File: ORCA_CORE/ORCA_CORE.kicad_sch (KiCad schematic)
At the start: 0 parts

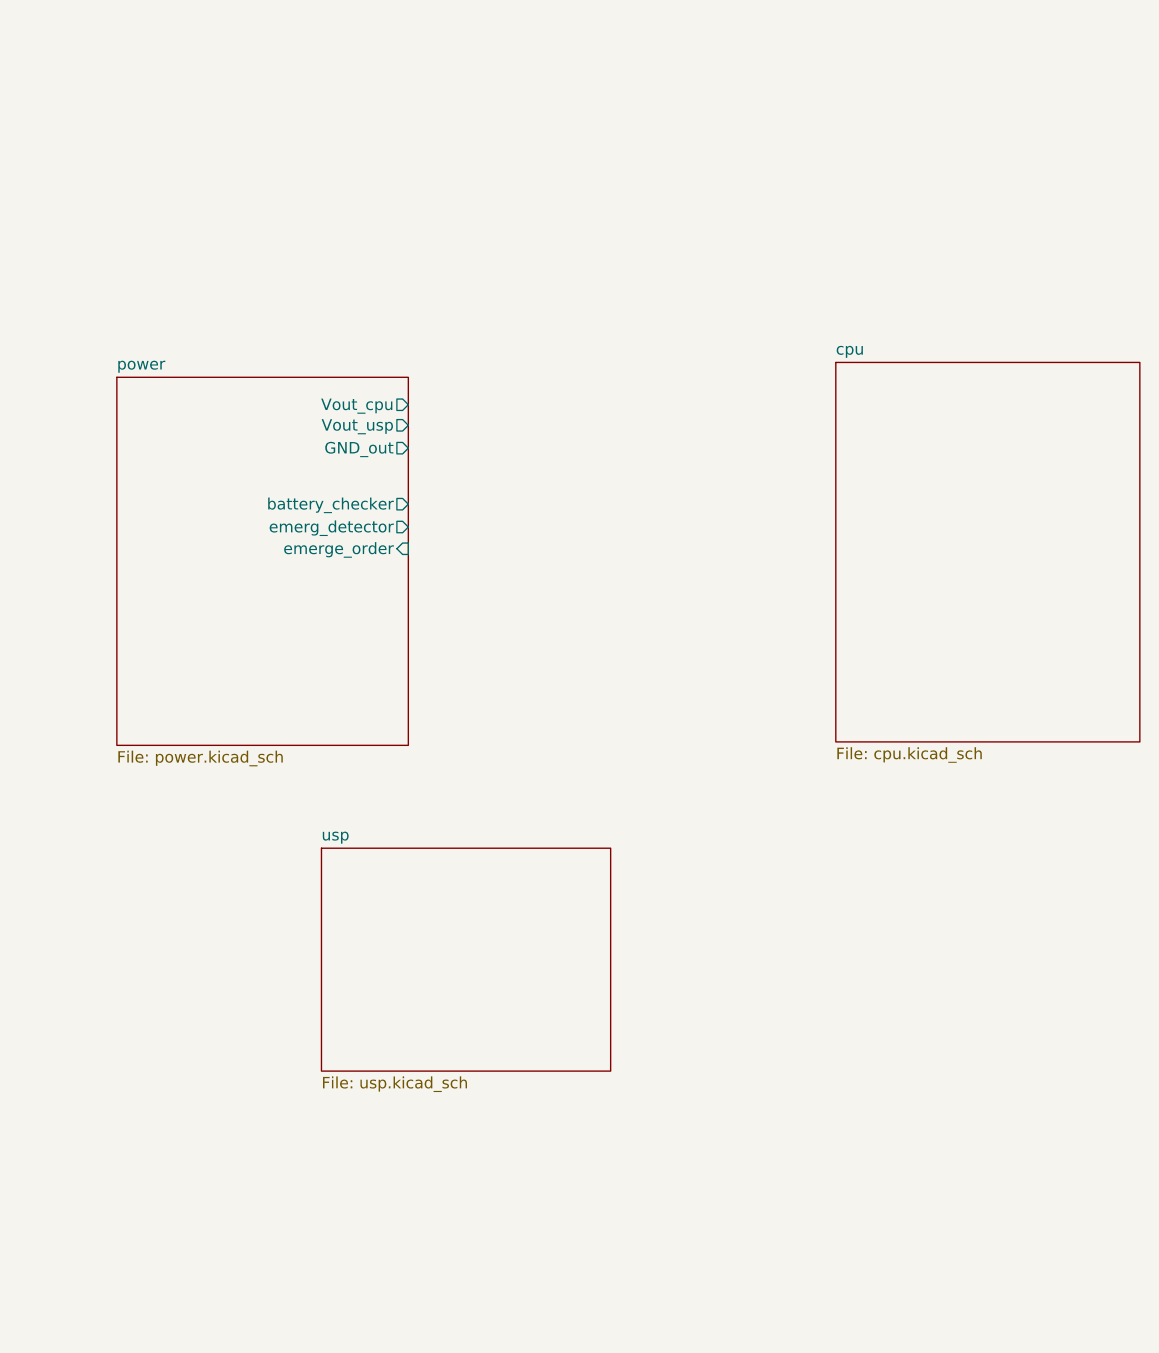
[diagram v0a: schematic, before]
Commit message: making usp
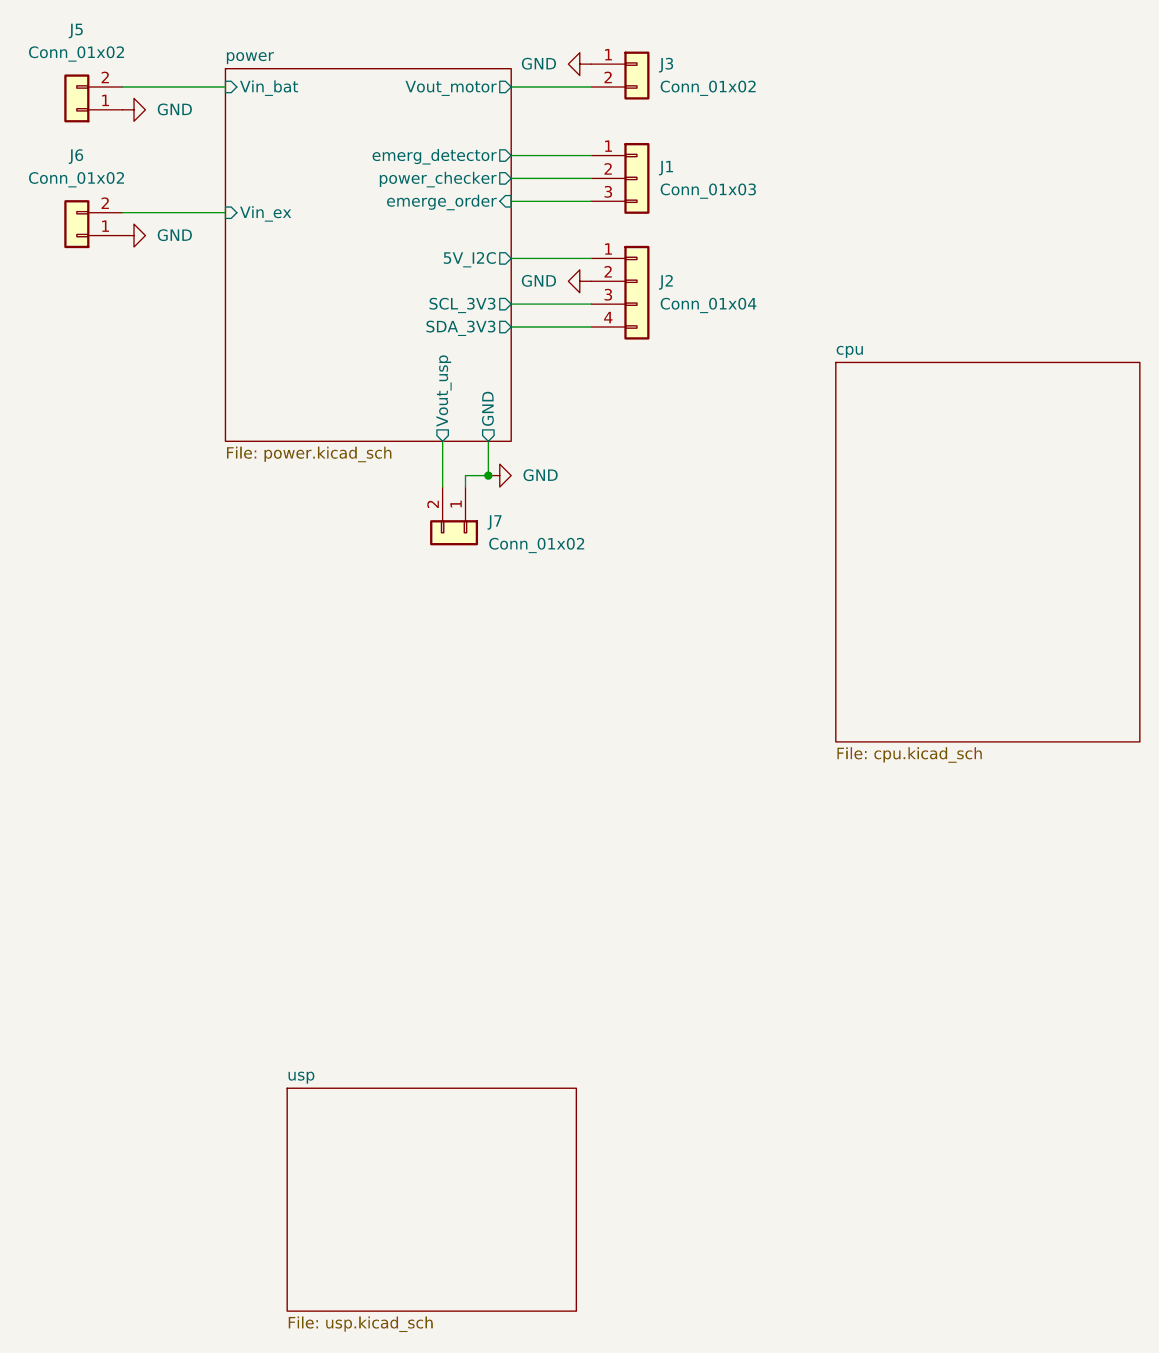
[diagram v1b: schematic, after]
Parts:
- added J1: Conn_01x03, symbol Connector_Generic:Conn_01x03
- added J2: Conn_01x04, symbol Connector_Generic:Conn_01x04
- added J3, J5, J6, J7: Conn_01x02, symbol Connector_Generic:Conn_01x02
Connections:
- net power/Vout_usp: now also J7.2 (Pin_2)
- net power/emerg_detector: now also J1.1 (Pin_1)
- net power/emerge_order: now also J1.3 (Pin_3)
- new net GND: J2.2 (Pin_2), J3.1 (Pin_1), J5.1 (Pin_1), J6.1 (Pin_1), J7.1 (Pin_1)
- new net power/5V_I2C: J2.1 (Pin_1)
- new net power/SCL_3V3: J2.3 (Pin_3)
- new net power/SDA_3V3: J2.4 (Pin_4)
- new net power/Vin_bat: J5.2 (Pin_2)
- new net power/Vin_ex: J6.2 (Pin_2)
- new net power/Vout_motor: J3.2 (Pin_2)
- new net power/power_checker: J1.2 (Pin_2)
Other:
- sheet power ports: added 5V_I2C, GND, SCL_3V3, SDA_3V3, Vin_bat, Vin_ex, Vout_motor, power_checker; removed GND_out, Vout_cpu, battery_checker
